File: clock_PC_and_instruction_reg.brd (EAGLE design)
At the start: 100 x 100 mm, 35 parts

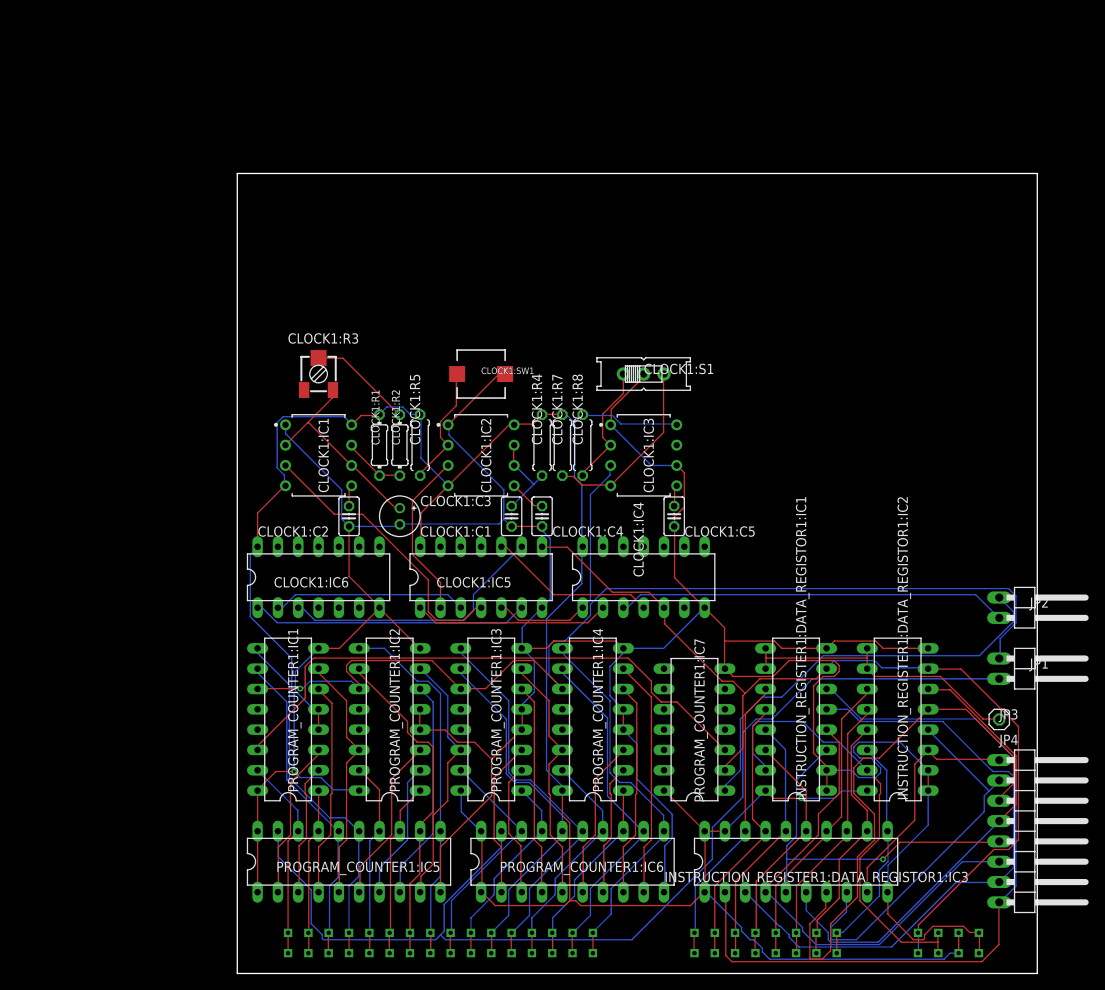
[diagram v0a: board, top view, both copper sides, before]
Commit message: Finished all design
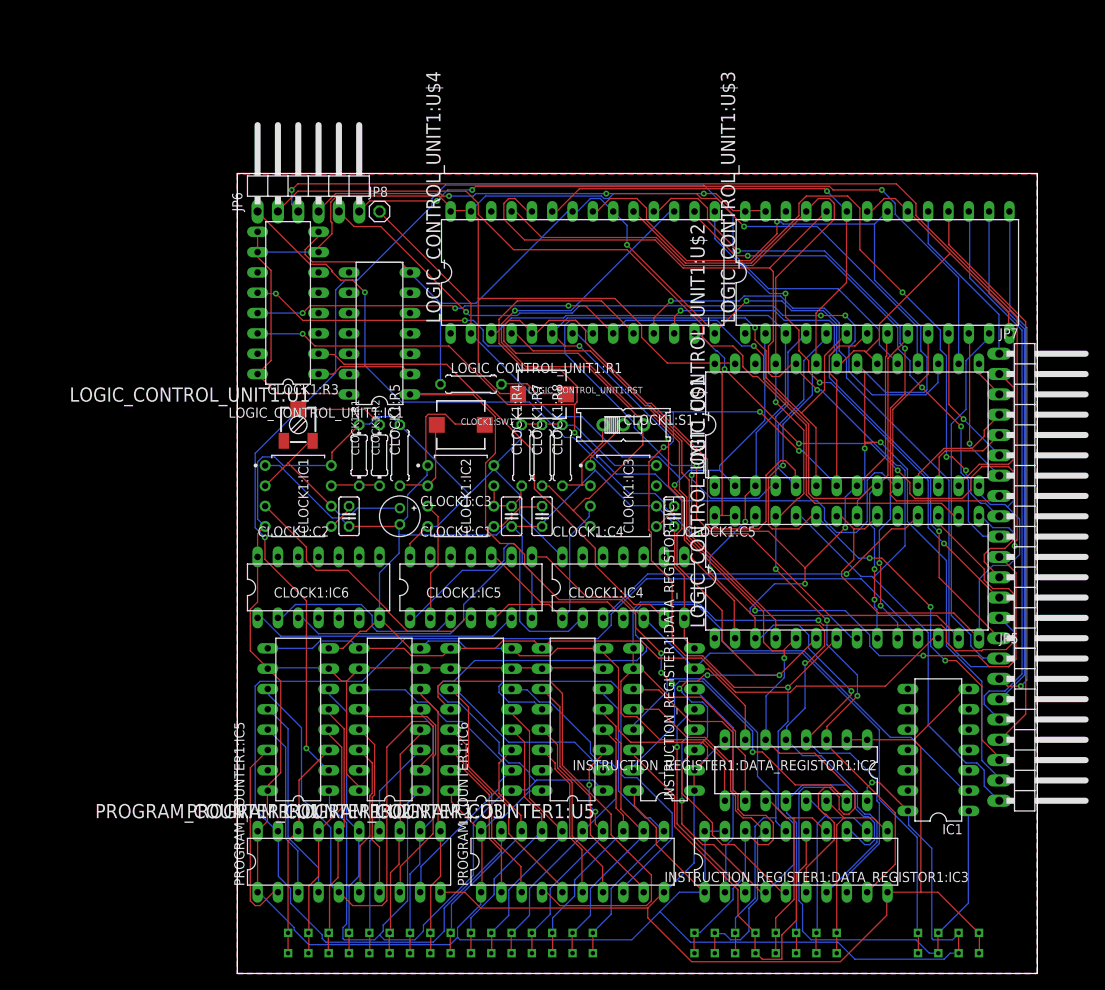
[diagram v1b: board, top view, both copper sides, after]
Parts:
- removed JP1, JP2: (no value), pinhead:1X02/90
- removed JP3: (no value), pinhead:1X01
- removed JP4: (no value), pinhead:1X08/90
- removed PROGRAM_COUNTER1:IC1, PROGRAM_COUNTER1:IC2, PROGRAM_COUNTER1:IC3, PROGRAM_COUNTER1:IC4: 74LS191N, 74xx-eu:DIL16
- removed PROGRAM_COUNTER1:IC7: 74LS08N, 74xx-eu:DIL14
- added IC1, LOGIC_CONTROL_UNIT1:IC1: 74LS04N, 74xx-eu:DIL14
- added JP5: (no value), pinhead:1X08/90
- added JP6: (no value), pinhead:1X06/90
- added JP7: (no value), pinhead:1X15/90
- added JP8: (no value), pinhead:1X01
- added LOGIC_CONTROL_UNIT1:R1: 1M, resistor:0207/7
- added LOGIC_CONTROL_UNIT1:RST: (no value), adafruit:PUSHBUTTON_SMD_SJ
- added LOGIC_CONTROL_UNIT1:U$1, LOGIC_CONTROL_UNIT1:U$2, LOGIC_CONTROL_UNIT1:U$3, LOGIC_CONTROL_UNIT1:U$4: AT28C256-28DIP, atmel-custom:DIL28-6
- added LOGIC_CONTROL_UNIT1:U1, PROGRAM_COUNTER1:U1, PROGRAM_COUNTER1:U2, PROGRAM_COUNTER1:U3, PROGRAM_COUNTER1:U5: 74LS161N, oldchips:DIL16
- moved INSTRUCTION_REGISTER1:DATA_REGISTOR1:IC1 16.5 mm to (-59.7, 33.0)
- moved INSTRUCTION_REGISTER1:DATA_REGISTOR1:IC2 14.2 mm to (-43.2, 26.7), turned to 180 degrees
- moved CLOCK1:SW1 6.84 mm to (-85.1, 69.8)
- moved CLOCK1:S1 6.84 mm to (-64.8, 69.8)
- moved CLOCK1:R3 6.84 mm to (-105.4, 69.8)
- moved CLOCK1:IC2 5.68 mm to (-85.1, 61.0)
- moved CLOCK1:IC3 5.68 mm to (-64.8, 61.0)
- moved CLOCK1:IC1 5.68 mm to (-105.4, 61.0)
- moved CLOCK1:R1 2.84 mm to (-97.8, 66.0)
- moved CLOCK1:R2 2.84 mm to (-95.2, 66.0)
- moved CLOCK1:R7 2.84 mm to (-74.9, 66.0)
- moved CLOCK1:R8 2.84 mm to (-72.4, 66.0)
- moved CLOCK1:IC4 2.84 mm to (-64.8, 49.5)
- moved CLOCK1:R4 2.84 mm to (-77.5, 66.0)
- moved CLOCK1:R5 2.84 mm to (-92.7, 66.0)
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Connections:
- removed net CLOCK1:!CLOCK: CLOCK1:IC4.6
- removed net PROGRAM_COUNTER1:PCA: PROGRAM_COUNTER1:IC1.14, PROGRAM_COUNTER1:IC7.3
- new net ADD: JP5.1, LOGIC_CONTROL_UNIT1:U$3.13
- new net AI: JP7.15, LOGIC_CONTROL_UNIT1:U$4.12
- new net AND: JP5.3, LOGIC_CONTROL_UNIT1:U$3.16
- new net AO: JP7.14, LOGIC_CONTROL_UNIT1:U$4.11
- new net BI: JP7.13, LOGIC_CONTROL_UNIT1:U$4.15
- new net BO: JP7.12, LOGIC_CONTROL_UNIT1:U$4.13
- new net CF: JP5.6, LOGIC_CONTROL_UNIT1:U$1.23, LOGIC_CONTROL_UNIT1:U$2.23, LOGIC_CONTROL_UNIT1:U$3.23, LOGIC_CONTROL_UNIT1:U$4.23
- new net CI: JP7.11, LOGIC_CONTROL_UNIT1:U$4.17
- new net CO: JP7.10, LOGIC_CONTROL_UNIT1:U$4.16
- new net D2A_HI_IN: JP6.6, LOGIC_CONTROL_UNIT1:U$2.16
- new net D2A_LO_IN: JP6.5, LOGIC_CONTROL_UNIT1:U$2.17
- new net D2A_OUT: JP6.4, LOGIC_CONTROL_UNIT1:U$2.18
- new net DI: JP7.9, LOGIC_CONTROL_UNIT1:U$4.19
- new net DO: JP7.8, LOGIC_CONTROL_UNIT1:U$4.18
- new net EI: JP7.7, LOGIC_CONTROL_UNIT1:U$3.12
- new net EO: JP7.6, LOGIC_CONTROL_UNIT1:U$3.11
- new net HI: JP7.5, LOGIC_CONTROL_UNIT1:U$2.12
- new net HL_TO_ADDR: JP7.1, LOGIC_CONTROL_UNIT1:U$3.19
- new net HO: JP7.4, LOGIC_CONTROL_UNIT1:U$2.11
- new net LI: JP7.3, LOGIC_CONTROL_UNIT1:U$2.15
- new net LO: JP7.2, LOGIC_CONTROL_UNIT1:U$2.13
- new net LOGIC_CONTROL_UNIT1:GND: LOGIC_CONTROL_UNIT1:IC1.7, LOGIC_CONTROL_UNIT1:R1.1, LOGIC_CONTROL_UNIT1:U$1.14, LOGIC_CONTROL_UNIT1:U$1.20, LOGIC_CONTROL_UNIT1:U$1.22, LOGIC_CONTROL_UNIT1:U$2.14, LOGIC_CONTROL_UNIT1:U$2.20, LOGIC_CONTROL_UNIT1:U$2.22, LOGIC_CONTROL_UNIT1:U$3.14, LOGIC_CONTROL_UNIT1:U$3.20, LOGIC_CONTROL_UNIT1:U$3.22, LOGIC_CONTROL_UNIT1:U$4.14, LOGIC_CONTROL_UNIT1:U$4.20, LOGIC_CONTROL_UNIT1:U$4.22, LOGIC_CONTROL_UNIT1:U1.8
- new net LOGIC_CONTROL_UNIT1:N$1: LOGIC_CONTROL_UNIT1:U$1.10, LOGIC_CONTROL_UNIT1:U$2.10, LOGIC_CONTROL_UNIT1:U$3.10, LOGIC_CONTROL_UNIT1:U$4.10, LOGIC_CONTROL_UNIT1:U1.14
- new net LOGIC_CONTROL_UNIT1:N$10: LOGIC_CONTROL_UNIT1:U$1.9, LOGIC_CONTROL_UNIT1:U$2.9, LOGIC_CONTROL_UNIT1:U$3.9, LOGIC_CONTROL_UNIT1:U$4.9, LOGIC_CONTROL_UNIT1:U1.13
- new net LOGIC_CONTROL_UNIT1:N$11: LOGIC_CONTROL_UNIT1:U$1.8, LOGIC_CONTROL_UNIT1:U$2.8, LOGIC_CONTROL_UNIT1:U$3.8, LOGIC_CONTROL_UNIT1:U$4.8, LOGIC_CONTROL_UNIT1:U1.12
- new net LOGIC_CONTROL_UNIT1:N$12: LOGIC_CONTROL_UNIT1:U1.11
- new net LOGIC_CONTROL_UNIT1:N$2: LOGIC_CONTROL_UNIT1:IC1.2, LOGIC_CONTROL_UNIT1:U1.1
- new net LOGIC_CONTROL_UNIT1:VCC: LOGIC_CONTROL_UNIT1:IC1.14, LOGIC_CONTROL_UNIT1:RST.P$2, LOGIC_CONTROL_UNIT1:U$1.27, LOGIC_CONTROL_UNIT1:U$1.28, LOGIC_CONTROL_UNIT1:U$2.27, LOGIC_CONTROL_UNIT1:U$2.28, LOGIC_CONTROL_UNIT1:U$3.27, LOGIC_CONTROL_UNIT1:U$3.28, LOGIC_CONTROL_UNIT1:U$4.27, LOGIC_CONTROL_UNIT1:U$4.28, LOGIC_CONTROL_UNIT1:U1.10, LOGIC_CONTROL_UNIT1:U1.16, LOGIC_CONTROL_UNIT1:U1.7, LOGIC_CONTROL_UNIT1:U1.9
- new net MAR_IN: JP6.1, LOGIC_CONTROL_UNIT1:U$1.13
- new net M_READ: JP6.2, LOGIC_CONTROL_UNIT1:U$1.16
- new net M_WRITE: JP6.3, LOGIC_CONTROL_UNIT1:U$1.15
- new net N$27: IC1.2, PROGRAM_COUNTER1:U1.1, PROGRAM_COUNTER1:U2.1, PROGRAM_COUNTER1:U3.1, PROGRAM_COUNTER1:U5.1
- new net N$34: CLOCK1:IC4.6, LOGIC_CONTROL_UNIT1:U1.2
- new net NF: JP5.7, LOGIC_CONTROL_UNIT1:U$1.21, LOGIC_CONTROL_UNIT1:U$2.21, LOGIC_CONTROL_UNIT1:U$3.21, LOGIC_CONTROL_UNIT1:U$4.21
- new net OR: JP5.4, LOGIC_CONTROL_UNIT1:U$3.17
- new net READY: JP8.1, LOGIC_CONTROL_UNIT1:U$1.2, LOGIC_CONTROL_UNIT1:U$2.2, LOGIC_CONTROL_UNIT1:U$3.2, LOGIC_CONTROL_UNIT1:U$4.2
- new net SUB: JP5.2, LOGIC_CONTROL_UNIT1:U$3.15
- new net XOR: JP5.5, LOGIC_CONTROL_UNIT1:U$3.18
- new net ZF: JP5.8, LOGIC_CONTROL_UNIT1:U$1.24, LOGIC_CONTROL_UNIT1:U$2.24, LOGIC_CONTROL_UNIT1:U$3.24, LOGIC_CONTROL_UNIT1:U$4.24
- net !II: now also LOGIC_CONTROL_UNIT1:U$1.17; no longer JP3.1
- net !PCL: now also LOGIC_CONTROL_UNIT1:U$1.12, PROGRAM_COUNTER1:U1.9, PROGRAM_COUNTER1:U2.9, PROGRAM_COUNTER1:U3.9, PROGRAM_COUNTER1:U5.9; no longer JP1.1, PROGRAM_COUNTER1:IC1.11, PROGRAM_COUNTER1:IC2.11, PROGRAM_COUNTER1:IC3.11, PROGRAM_COUNTER1:IC4.11
- net !PCO: now also LOGIC_CONTROL_UNIT1:U$1.11; no longer JP1.2
- net GND: now also IC1.7, PROGRAM_COUNTER1:U1.8, PROGRAM_COUNTER1:U2.8, PROGRAM_COUNTER1:U3.8, PROGRAM_COUNTER1:U5.8; no longer PROGRAM_COUNTER1:IC1.4, PROGRAM_COUNTER1:IC1.5, PROGRAM_COUNTER1:IC1.8, PROGRAM_COUNTER1:IC2.4, PROGRAM_COUNTER1:IC2.5, PROGRAM_COUNTER1:IC2.8, PROGRAM_COUNTER1:IC3.4, PROGRAM_COUNTER1:IC3.5, PROGRAM_COUNTER1:IC3.8, PROGRAM_COUNTER1:IC4.4, PROGRAM_COUNTER1:IC4.5, PROGRAM_COUNTER1:IC4.8, PROGRAM_COUNTER1:IC7.7
- net HALT: now also LOGIC_CONTROL_UNIT1:U$1.18; no longer JP2.2
- net IRO0: no longer JP4.8
- net IRO7: now also LOGIC_CONTROL_UNIT1:U$1.25, LOGIC_CONTROL_UNIT1:U$2.25, LOGIC_CONTROL_UNIT1:U$3.25, LOGIC_CONTROL_UNIT1:U$4.25; no longer JP4.1
- net N$1: now also PROGRAM_COUNTER1:U5.6; no longer PROGRAM_COUNTER1:IC4.9
- net N$10: now also PROGRAM_COUNTER1:U2.5; no longer PROGRAM_COUNTER1:IC2.10
- net N$11: now also PROGRAM_COUNTER1:U2.4; no longer PROGRAM_COUNTER1:IC2.1
- net N$12: now also PROGRAM_COUNTER1:U2.3; no longer PROGRAM_COUNTER1:IC2.15
- net N$13: now also PROGRAM_COUNTER1:U1.6; no longer PROGRAM_COUNTER1:IC1.9
- net N$14: now also PROGRAM_COUNTER1:U1.5; no longer PROGRAM_COUNTER1:IC1.10
- net N$15: now also PROGRAM_COUNTER1:U1.4; no longer PROGRAM_COUNTER1:IC1.1
- net N$16: now also PROGRAM_COUNTER1:U1.3; no longer PROGRAM_COUNTER1:IC1.15
- net N$2: now also PROGRAM_COUNTER1:U5.5; no longer PROGRAM_COUNTER1:IC4.10
- net N$25: no longer PROGRAM_COUNTER1:IC7.2
- net N$26: now also IC1.1, LOGIC_CONTROL_UNIT1:IC1.1, LOGIC_CONTROL_UNIT1:R1.2, LOGIC_CONTROL_UNIT1:RST.P$1
- net N$28: now also LOGIC_CONTROL_UNIT1:U$1.3, LOGIC_CONTROL_UNIT1:U$2.3, LOGIC_CONTROL_UNIT1:U$3.3, LOGIC_CONTROL_UNIT1:U$4.3; no longer JP4.2
- net N$29: now also LOGIC_CONTROL_UNIT1:U$1.4, LOGIC_CONTROL_UNIT1:U$2.4, LOGIC_CONTROL_UNIT1:U$3.4, LOGIC_CONTROL_UNIT1:U$4.4; no longer JP4.3
- net N$3: now also PROGRAM_COUNTER1:U5.4; no longer PROGRAM_COUNTER1:IC4.1
- net N$30: now also LOGIC_CONTROL_UNIT1:U$1.5, LOGIC_CONTROL_UNIT1:U$2.5, LOGIC_CONTROL_UNIT1:U$3.5, LOGIC_CONTROL_UNIT1:U$4.5; no longer JP4.4
- net N$31: now also LOGIC_CONTROL_UNIT1:U$1.6, LOGIC_CONTROL_UNIT1:U$2.6, LOGIC_CONTROL_UNIT1:U$3.6, LOGIC_CONTROL_UNIT1:U$4.6; no longer JP4.5
- net N$32: now also LOGIC_CONTROL_UNIT1:U$1.7, LOGIC_CONTROL_UNIT1:U$2.7, LOGIC_CONTROL_UNIT1:U$3.7, LOGIC_CONTROL_UNIT1:U$4.7; no longer JP4.6
- net N$33: no longer JP4.7
- net N$4: now also PROGRAM_COUNTER1:U5.3; no longer PROGRAM_COUNTER1:IC4.15
- net N$5: now also PROGRAM_COUNTER1:U3.6; no longer PROGRAM_COUNTER1:IC3.9
- net N$6: now also PROGRAM_COUNTER1:U3.5; no longer PROGRAM_COUNTER1:IC3.10
- net N$7: now also PROGRAM_COUNTER1:U3.4; no longer PROGRAM_COUNTER1:IC3.1
- net N$8: now also PROGRAM_COUNTER1:U3.3; no longer PROGRAM_COUNTER1:IC3.15
- net N$9: now also PROGRAM_COUNTER1:U2.6; no longer PROGRAM_COUNTER1:IC2.9
- net PC_AD: now also LOGIC_CONTROL_UNIT1:U$2.19, PROGRAM_COUNTER1:U1.2; no longer JP2.1, PROGRAM_COUNTER1:IC7.1
- net PROGRAM_COUNTER1:N$2: now also PROGRAM_COUNTER1:U1.11, PROGRAM_COUNTER1:U2.2; no longer PROGRAM_COUNTER1:IC1.7, PROGRAM_COUNTER1:IC2.14
- net PROGRAM_COUNTER1:N$23: now also PROGRAM_COUNTER1:U1.14; no longer PROGRAM_COUNTER1:IC1.3
- net PROGRAM_COUNTER1:N$24: now also PROGRAM_COUNTER1:U1.13; no longer PROGRAM_COUNTER1:IC1.2
- net PROGRAM_COUNTER1:N$25: now also PROGRAM_COUNTER1:U1.12; no longer PROGRAM_COUNTER1:IC1.6
- net PROGRAM_COUNTER1:N$26: now also PROGRAM_COUNTER1:U2.14; no longer PROGRAM_COUNTER1:IC2.3
- net PROGRAM_COUNTER1:N$27: now also PROGRAM_COUNTER1:U2.13; no longer PROGRAM_COUNTER1:IC2.2
- net PROGRAM_COUNTER1:N$28: now also PROGRAM_COUNTER1:U2.12; no longer PROGRAM_COUNTER1:IC2.6
- net PROGRAM_COUNTER1:N$3: now also PROGRAM_COUNTER1:U2.11, PROGRAM_COUNTER1:U3.2; no longer PROGRAM_COUNTER1:IC2.7, PROGRAM_COUNTER1:IC3.14
- net PROGRAM_COUNTER1:N$30: now also PROGRAM_COUNTER1:U3.14; no longer PROGRAM_COUNTER1:IC3.3
- net PROGRAM_COUNTER1:N$31: now also PROGRAM_COUNTER1:U3.13; no longer PROGRAM_COUNTER1:IC3.2
- net PROGRAM_COUNTER1:N$32: now also PROGRAM_COUNTER1:U3.12; no longer PROGRAM_COUNTER1:IC3.6
- net PROGRAM_COUNTER1:N$34: now also PROGRAM_COUNTER1:U5.14; no longer PROGRAM_COUNTER1:IC4.3
- net PROGRAM_COUNTER1:N$35: now also PROGRAM_COUNTER1:U5.13; no longer PROGRAM_COUNTER1:IC4.2
- net PROGRAM_COUNTER1:N$36: now also PROGRAM_COUNTER1:U5.12; no longer PROGRAM_COUNTER1:IC4.6
- net PROGRAM_COUNTER1:N$37: now also PROGRAM_COUNTER1:U5.11; no longer PROGRAM_COUNTER1:IC4.7
- net PROGRAM_COUNTER1:N$4: now also PROGRAM_COUNTER1:U3.11, PROGRAM_COUNTER1:U5.2; no longer PROGRAM_COUNTER1:IC3.7, PROGRAM_COUNTER1:IC4.14
- net VCC: now also IC1.14, PROGRAM_COUNTER1:U1.10, PROGRAM_COUNTER1:U1.16, PROGRAM_COUNTER1:U1.7, PROGRAM_COUNTER1:U2.10, PROGRAM_COUNTER1:U2.16, PROGRAM_COUNTER1:U2.7, PROGRAM_COUNTER1:U3.10, PROGRAM_COUNTER1:U3.16, PROGRAM_COUNTER1:U3.7, PROGRAM_COUNTER1:U5.10, PROGRAM_COUNTER1:U5.16, PROGRAM_COUNTER1:U5.7; no longer PROGRAM_COUNTER1:IC1.16, PROGRAM_COUNTER1:IC2.16, PROGRAM_COUNTER1:IC3.16, PROGRAM_COUNTER1:IC4.16, PROGRAM_COUNTER1:IC7.14
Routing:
- net LOGIC_CONTROL_UNIT1:GND: track 0.00 -> 235.7 mm, vias 0 -> 2
- net N$27: track 0.00 -> 190.4 mm
- net LOGIC_CONTROL_UNIT1:VCC: track 0.00 -> 190.0 mm, vias 0 -> 1
- net LOGIC_CONTROL_UNIT1:N$1: track 0.00 -> 179.2 mm, vias 0 -> 4
- net LOGIC_CONTROL_UNIT1:N$11: track 0.00 -> 154.3 mm, vias 0 -> 5
- net ZF: track 0.00 -> 152.7 mm, vias 0 -> 1
- net NF: track 0.00 -> 149.4 mm, vias 0 -> 3
- net N$30: track 58.4 -> 200.6 mm, vias 0 -> 1
- net M_WRITE: track 0.00 -> 137.5 mm, vias 0 -> 2
- net LOGIC_CONTROL_UNIT1:N$10: track 0.00 -> 137.4 mm, vias 0 -> 6
- net CI: track 0.00 -> 132.5 mm, vias 0 -> 3
- net CF: track 0.00 -> 132.0 mm, vias 0 -> 5
- net N$26: track 55.9 -> 186.4 mm, vias 0 -> 4
- net N$31: track 47.5 -> 175.1 mm, vias 1 -> 6
- net IRO7: track 30.3 -> 150.3 mm, vias 0 -> 4
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- added copper zone on layer 1, net GND
- added copper zone on layer 16, net GND
